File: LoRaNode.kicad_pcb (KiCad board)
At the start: 2 copper layers, 43 x 93 mm, 59 parts, among them J10 D4, J11 A1, J12 A2, J13 A3, J14 D8, J2 Conn_01x06, J3 Conn_01x02, J4 ISP, J5 Conn_01x06, J6 Conn_01x04, J7 USB_B_Micro, J8 D2, J9 D3, U1 RFM95W-868S2, U2 MCP73871, U3 TPS63031, U4 ATMEGA328P-AU, Y1 8MHz HC5032/4

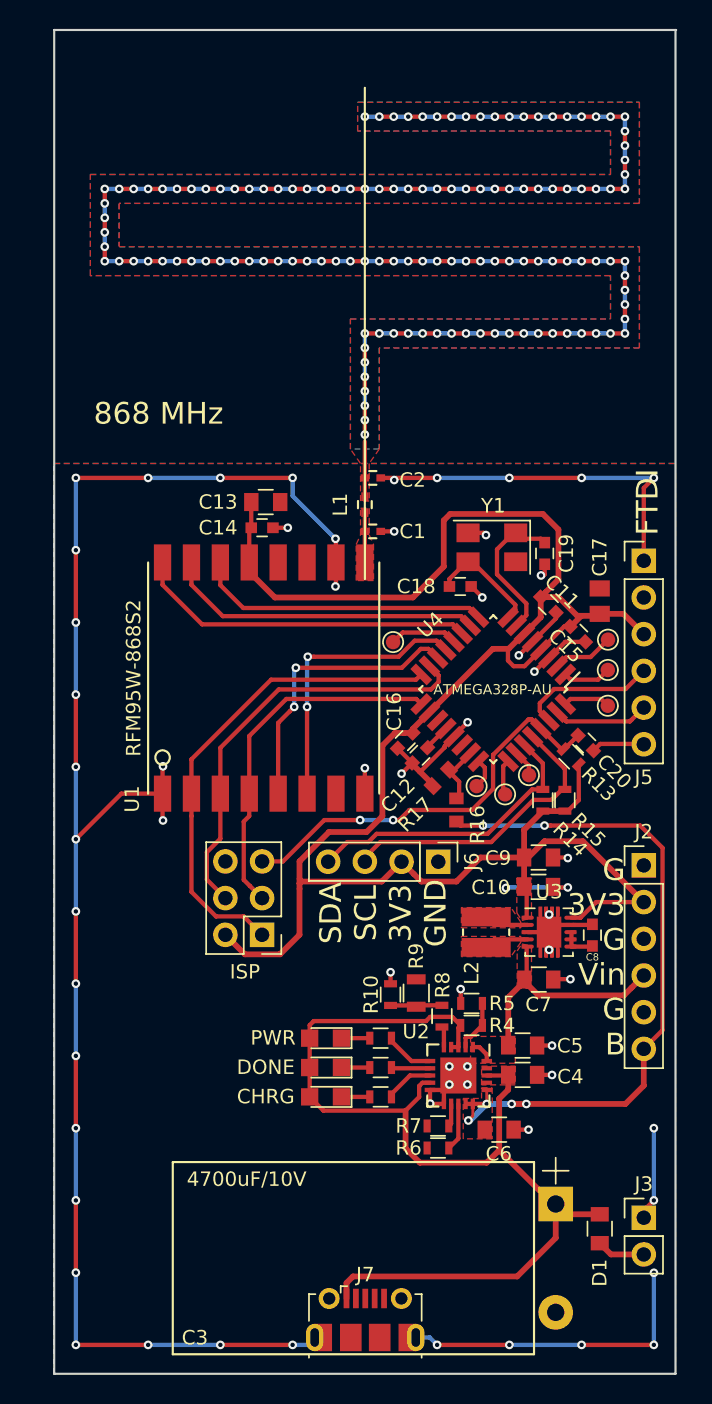
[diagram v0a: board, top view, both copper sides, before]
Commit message: v0.1
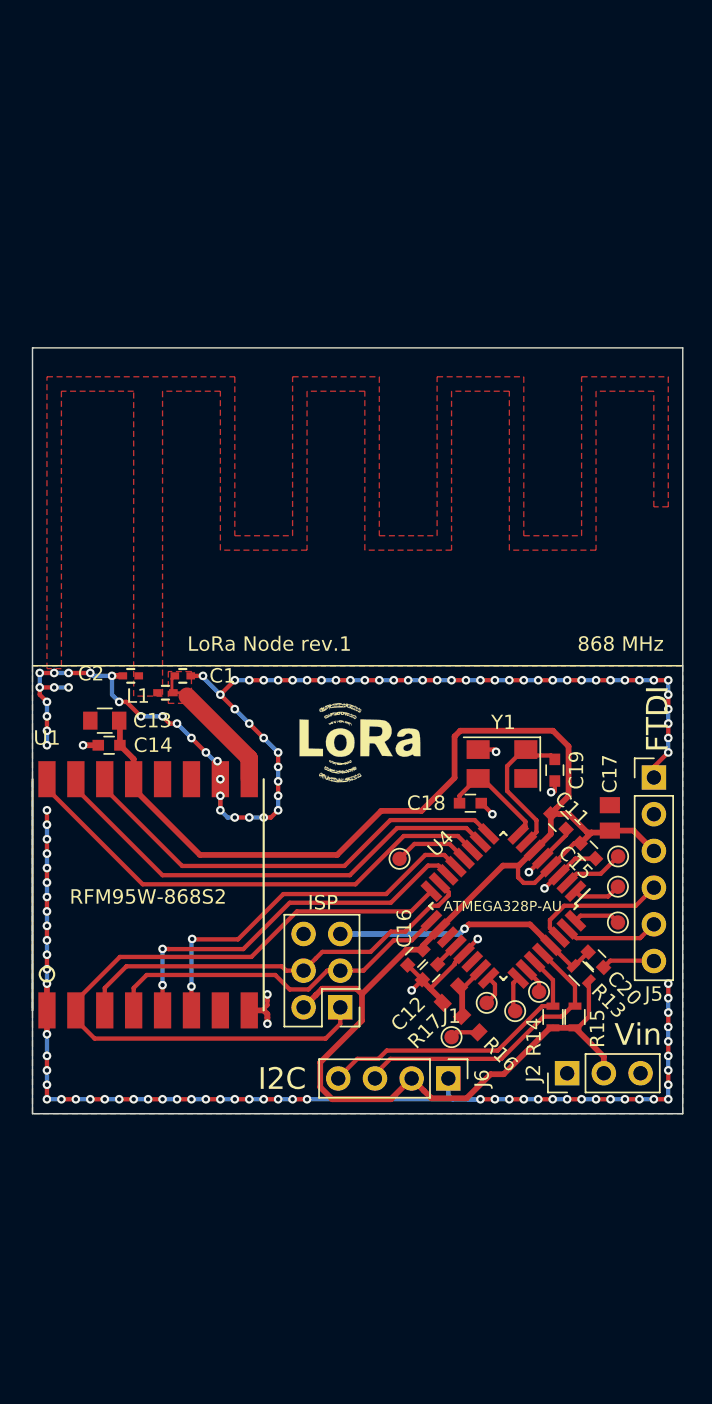
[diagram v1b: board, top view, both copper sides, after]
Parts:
- removed C10, C4, C5, C6, C7, C9: 10u, Capacitors_SMD:C_0805
- removed C3: 4700uF/10V, Capacitors_THT:CP_Radial_D12.5mm_P25mm
- removed C8: 100n, Capacitors_SMD:C_0603
- removed D1: MBR120VLSFT1G, Capacitors_SMD:C_0805
- removed D2: CHRG, LEDs:LED_0805
- removed D3: DONE, LEDs:LED_0805
- removed D4: PWR, LEDs:LED_0805
- removed J3: Conn_01x02, Pin_Headers:Pin_Header_Straight_1x02_Pitch2.54mm
- removed J7: USB_B_Micro, Connector_USB:USB_Micro-B_Molex-105017-0001
- removed L2: 1u5, Inductors:Inductor_Wurth_MAPI-3012
- removed R1, R2, R3: 1k, Resistors_SMD:R_0603
- removed R10: 69k8, Resistors_SMD:R_0603
- removed R4: 270k, Resistors_SMD:R_0603
- removed R5, R7: 100k, Resistors_SMD:R_0603
- removed R6: 2k, Resistors_SMD:R_0603
- removed R8: 1k54, Resistors_SMD:R_0603
- removed R9: THERM 10k, Resistors_SMD:R_0805
- removed U2: MCP73871, Housings_DFN_QFN:QFN-20-1EP_4x4mm_Pitch0.5mm
- removed U3: TPS63031, Package_SON:Texas_S-PWSON-N10
- added G***: LoRa-Logo-Small, kicad-footprints-master:LoRa-Logo-Small, F.Cu at (150.1, 93.7)
- added G***: RiskeLogo, kicad-footprints-master:RiskeLogo, B.Cu at (136.0, 94.7)
- added J1: A3, TestPoint:TestPoint_Pad_D1.0mm, F.Cu at (156.0, 113.7)
- added openhw: , kicad-footprints-master:openhw, B.Cu at (142.4, 106.4)
- C1: value 2p7 -> dnp
- J2: value Conn_01x06 -> Conn_01x03; footprint Pin_Headers:Pin_Header_Straight_1x06_Pitch2.54mm -> Connector_PinHeader_2.54mm:PinHeader_1x03_P2.54mm_Vertical
- L1: value 1n8 -> 0R
- moved C2 21.6 mm to (133.8, 88.7), turned to 180 degrees
- moved L1 19.0 mm to (136.2, 89.9), turned to 180 degrees
- moved C13 18.8 mm to (132.0, 91.8), turned to 180 degrees
- moved C14 18.4 mm to (132.3, 93.5), turned to 180 degrees
- moved U1 17.0 mm to (135.0, 103.8)
- moved C1 16.5 mm to (137.4, 88.7)
- moved J2 15.3 mm to (164.0, 116.2), turned to 90 degrees
- moved C11 15.0 mm to (163.4, 98.8)
- moved C12 15.0 mm to (154.5, 109.2)
- moved C15 15.0 mm to (165.4, 100.8)
- moved C16 15.0 mm to (153.5, 108.2)
- moved C17 15.0 mm to (167.0, 98.5)
- moved C18 15.0 mm to (157.3, 97.5)
- moved C19 15.0 mm to (163.1, 95.2)
- moved C20 15.0 mm to (166.0, 108.3)
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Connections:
- C1 pad 2: Earth -> GND
- C11 pad 2: Earth -> GND
- C12 pad 2: Earth -> GND
- C13 pad 2: Earth -> GND
- C14 pad 2: Earth -> GND
- C15 pad 2: Earth -> GND
- C16 pad 2: Earth -> GND
- C17 pad 2: Earth -> GND
- C18 pad 2: Earth -> GND
- C19 pad 2: Earth -> GND
- C2 pad 2: Earth -> GND
- J2 pad 1: Earth -> GND
- J2 pad 3: Earth -> GND
- J4 pad 6: Earth -> GND
- J5 pad 1: Earth -> GND
- J5 pad 2: Earth -> GND
- J6 pad 1: Earth -> GND
- R17 pad 2: Earth -> GND
- U1 pad 1: Earth -> GND
- U1 pad 10: Earth -> GND
- U1 pad 8: Earth -> GND
- U4 pad 21: Earth -> GND
- U4 pad 3: Earth -> GND
- U4 pad 5: Earth -> GND
- Y1 pad 2: Earth -> GND
- Y1 pad 4: Earth -> GND
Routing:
- net Earth: track 212.7 -> 0.00 mm, vias 61 -> 0
- net GND: track 0.00 -> 185.3 mm, vias 0 -> 139
- net /ANT: track 133.8 -> 0.00 mm, vias 131 -> 0
- net VCC: track 73.1 -> 0.00 mm
- net /VBAT: track 49.7 -> 2.00 mm, vias 6 -> 0
- net /VOUT: track 18.7 -> 0.00 mm
- net /12(**/MOSI): track 33.6 -> 49.5 mm
- net +3V3: track 139.1 -> 124.4 mm
- net /D7: track 23.7 -> 34.6 mm
- net /D6: track 22.0 -> 32.9 mm
- net /D5: track 20.4 -> 31.1 mm
- net /RES: track 28.6 -> 19.0 mm, vias 2 -> 1
- net /10(**/SS): track 19.8 -> 26.6 mm
- net Net-(C1-Pad1): track 3.45 -> 9.83 mm
- net /D9: track 20.5 -> 26.7 mm
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- added copper zone on B.Cu, net GND
- added copper zone on F.Cu, net GND
- removed copper zone on F.Cu, net +3V3
- removed copper zone on B.Cu, net /ANT
- removed copper zone on F.Cu, net /VBAT
- removed copper zone on F.Cu, net /VOUT
- removed copper zone on B.Cu, net Earth
- removed copper zone on F.Cu, net Earth
- removed copper zone on F.Cu, net Net-(L2-Pad1)
- removed copper zone on F.Cu, net Net-(L2-Pad2)
- removed copper zone on F.Cu, net VCC
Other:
- board size 43 x 93 mm -> 45 x 53 mm
- net class Default: clearance 0.1 -> 0.25
- rule trace_clearance: 0.1 -> 0.25
- board text added: "GND 3V3 GND"
- board text added: "GND CTS 3V3 RX TX DTR"
- board text added: "I2C"
- board text added: "LoRa Node rev.1"
- board text added: "Vin"
- board text removed: "+ -"
- board text removed: "6V Solar panel"
- board text removed: "G 3V3 G Vin G B"
- board text removed: "GND - 3V3 RX TX RES"
- board text removed: "GND 3V3 GND VIN-6Vmax GND VBAT"
